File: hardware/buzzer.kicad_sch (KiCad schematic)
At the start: 4 parts, among them Q2 BC847

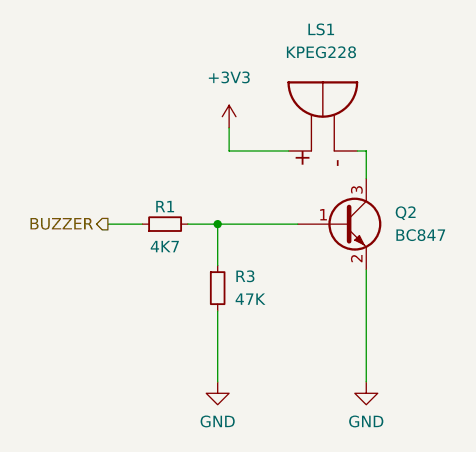
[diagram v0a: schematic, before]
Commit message: name stardandi added, readme file updated
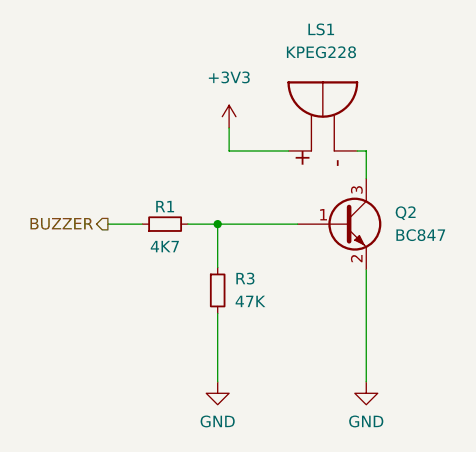
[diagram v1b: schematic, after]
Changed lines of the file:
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@@
     (stroke (width 0) (type default) (color 0 0 0 0))
   )
-  (wire (pts (xy 139.7 101.346) (xy 139.7 105.918))
+  (wire (pts (xy 139.7 101.346) (xy 139.7 106.172))
     (stroke (width 0) (type default) (color 0 0 0 0))
   )
@@
     (stroke (width 0) (type default) (color 0 0 0 0))
   )
-  (wire (pts (xy 139.7 110.998) (xy 139.7 118.872))
+  (wire (pts (xy 139.7 111.252) (xy 139.7 118.872))
     (stroke (width 0) (type default) (color 0 0 0 0))
   )
@@
     (pin "1")
   )
-  (symbol (lib_id "Device:R_Small") (at 139.7 108.458 0) (unit 1)
+  (symbol (lib_id "Device:R_Small") (at 139.7 108.712 0) (unit 1)
     (in_bom yes) (on_board yes) (fields_autoplaced)
-    (property "Reference" "R3" (id 0) (at 141.605 107.1879 0)
+    (property "Reference" "R3" (id 0) (at 141.605 107.4419 0)
       (effects (font (size 1.27 1.27)) (justify left))
     )
-    (property "Value" "47K" (id 1) (at 141.605 109.7279 0)
+    (property "Value" "47K" (id 1) (at 141.605 109.9819 0)
       (effects (font (size 1.27 1.27)) (justify left))
     )
-    (property "Footprint" "Resistor_SMD:R_0603_1608Metric" (id 2) (at 139.7 108.458 0)
+    (property "Footprint" "Resistor_SMD:R_0603_1608Metric" (id 2) (at 139.7 108.712 0)
       (effects (font (size 1.27 1.27)) hide)
     )
-    (property "Datasheet" "~" (id 3) (at 139.7 108.458 0)
+    (property "Datasheet" "~" (id 3) (at 139.7 108.712 0)
       (effects (font (size 1.27 1.27)) hide)
     )
